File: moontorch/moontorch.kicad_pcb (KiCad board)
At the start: 2 copper layers, 24.5 x 101 mm, 27 parts, among them J1 Conn_Coaxial, J2 Pogo_VLED_1, J3 Pogo_VLED_2, J4 BAT, J5 Torchbutton, J6 UART, J7 USB, J8 Pogo_GND, Q1 AP2317SD, SW3 RESET, SW4 BOOT, U1 HT-CT62, U2 L80-R, U3 XTX XTP2038-330AS2CT

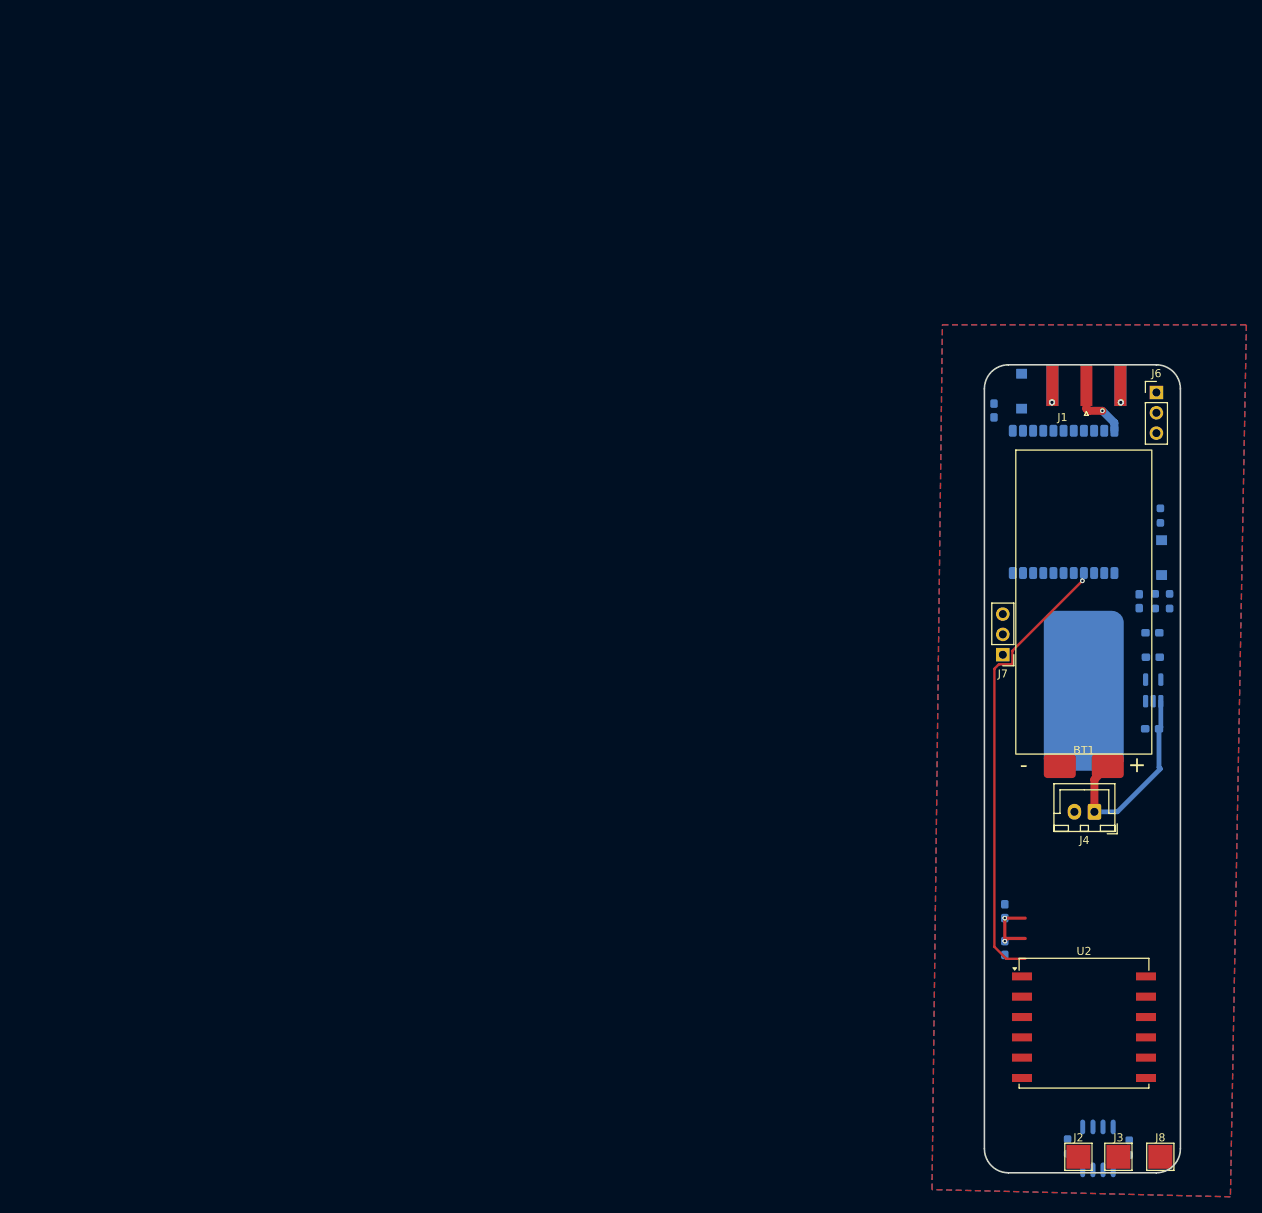
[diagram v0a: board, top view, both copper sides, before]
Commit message: weiter moontorch
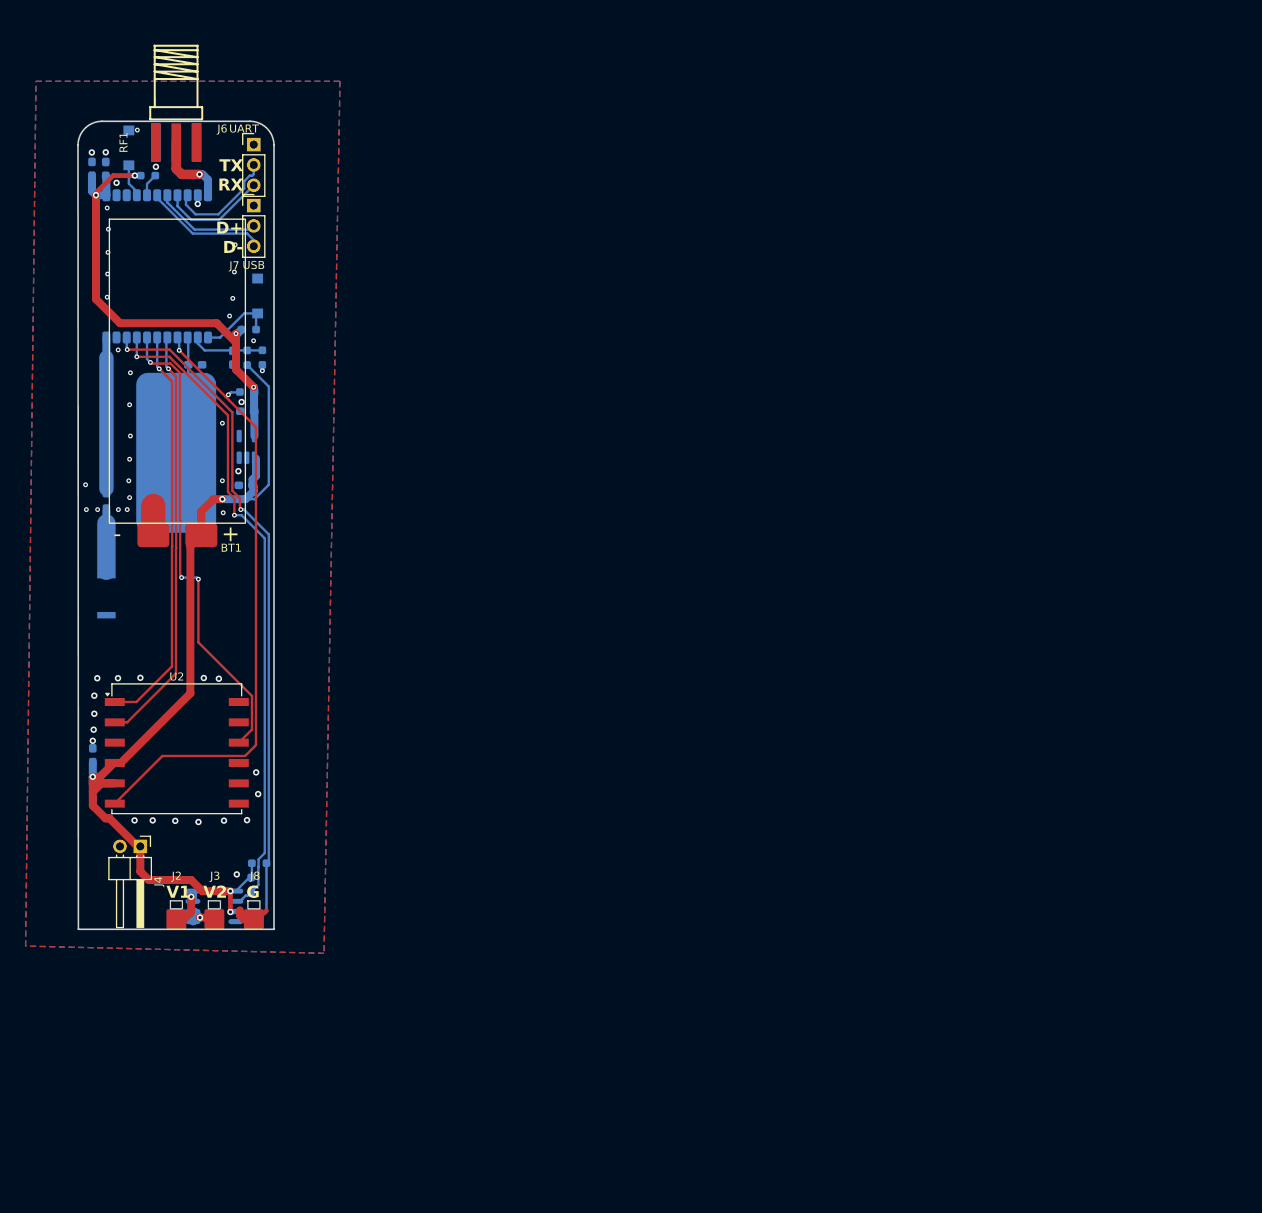
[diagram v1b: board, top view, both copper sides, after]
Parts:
- removed J1: Conn_Coaxial, Connector_Coaxial:SMA_Amphenol_132289_EdgeMount
- added C8: 1u, Capacitor_SMD:C_0603_1608Metric_Pad1.08x0.95mm_HandSolder, B.Cu at (103.4, 33.5)
- added R6: 0R, Resistor_SMD:R_0603_1608Metric_Pad0.98x0.95mm_HandSolder, B.Cu at (103.5, 75.0)
- added R8: 10K, Resistor_SMD:R_0603_1608Metric_Pad0.98x0.95mm_HandSolder, B.Cu at (108.7, 34.4)
- added R9: 10K, Resistor_SMD:R_0603_1608Metric_Pad0.98x0.95mm_HandSolder, B.Cu at (121.1, 61.4)
- added RF1: 443MHz, EasyEDA:SMA-SMD_BWSMA-KE-P001, F.Cu at (112.2, 30.2)
- added U4: 2.4GHz, EasyEDA:ANT-SMD_L5.0-W2.0, B.Cu at (103.5, 86.8)
- J2, J3, J8: footprint TestPoint:TestPoint_Pad_3.0x3.0mm -> hacrafu:Pogo Pin 3015
- J4: footprint Connector_JST:JST_XH_B2B-XH-A_1x02_P2.50mm_Vertical -> Connector_PinHeader_2.54mm:PinHeader_1x02_P2.54mm_Horizontal
- moved C7 124.3 mm to (114.6, 58.0), turned to 0 degrees
- moved R3 120.0 mm to (121.3, 53.6), turned to 180 degrees
- moved J4 119.3 mm to (107.7, 118.2), turned to -90 degrees
- moved U2 118.5 mm to (112.3, 106.0)
- moved SW3 117.6 mm to (122.4, 49.4)
- moved R4 117.5 mm to (121.1, 57.1)
- moved J8 117.5 mm to (121.9, 126.0)
- moved C1 117.3 mm to (120.9, 73.1)
- moved C3 117.3 mm to (119.3, 57.1)
- moved U3 117.3 mm to (121.0, 68.3)
- moved C2 117.3 mm to (121.1, 63.8)
- moved J5 117.3 mm to (112.2, 69.0)
- moved J3 117.2 mm to (117.0, 126.0)
- moved U1 117.1 mm to (109.8, 45.7)
- moved J6 117.0 mm to (121.9, 30.5)
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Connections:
- net Net-(J6-Pin_2) renamed /UART_TX
- net Net-(J6-Pin_3) renamed /UART_RX
- J7 pad 2: Net-(J7-Pin_2) -> /USB_DP
- J7 pad 3: Net-(J7-Pin_3) -> /USB_DN
- U1 pad 1: unconnected-(U1-2.4G_Ant-Pad1) -> Net-(U1-2.4G_Ant)
- U1 pad 16: unconnected-(U1-GPIO8-Pad16) -> Net-(U1-GPIO8)
- U1 pad 17: Net-(J7-Pin_2) -> /USB_DN
- U1 pad 18: Net-(J7-Pin_3) -> /USB_DP
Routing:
- net /LED2: track 0.00 -> 86.8 mm, vias 0 -> 2
- net /VBAT: track 33.6 -> 118.3 mm, vias 2 -> 4
- net /LED1: track 0.00 -> 82.0 mm, vias 0 -> 2
- net +3V3: track 0.00 -> 60.7 mm, vias 0 -> 4
- net /GPS_RESET: track 0.00 -> 59.4 mm, vias 0 -> 3
- net /GPS_TX: track 0.00 -> 52.7 mm, vias 0 -> 1
- net /GPS_RX: track 0.00 -> 50.9 mm, vias 0 -> 1
- net /GPS_PPS: track 56.6 -> 77.7 mm, vias 1 -> 2
- net Net-(U1-2.4G_Ant): track 0.00 -> 18.9 mm
- net /USB_DN: track 0.00 -> 15.4 mm
- net Net-(J5-Pin_1): track 0.00 -> 15.1 mm
- net /UART_TX: track 0.00 -> 14.0 mm
- net /UART_RX: track 0.00 -> 13.4 mm
- net /USB_DP: track 0.00 -> 13.3 mm
- net /RESET: track 0.00 -> 9.54 mm
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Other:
- outline, holes or cut-outs redrawn
- board text added: "D+ D-"
- board text added: "G"
- board text added: "TX RX"
- board text added: "V1"
- board text added: "V2"

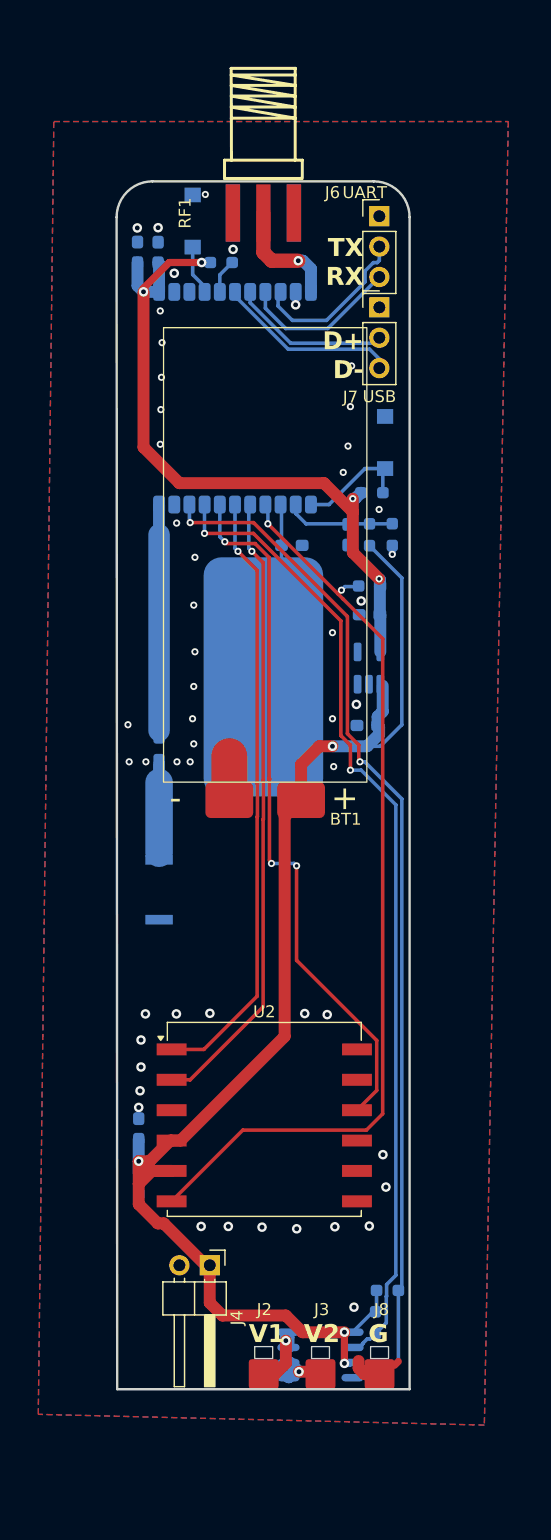
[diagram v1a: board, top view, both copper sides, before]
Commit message: zwischenstand bestellfähig 1
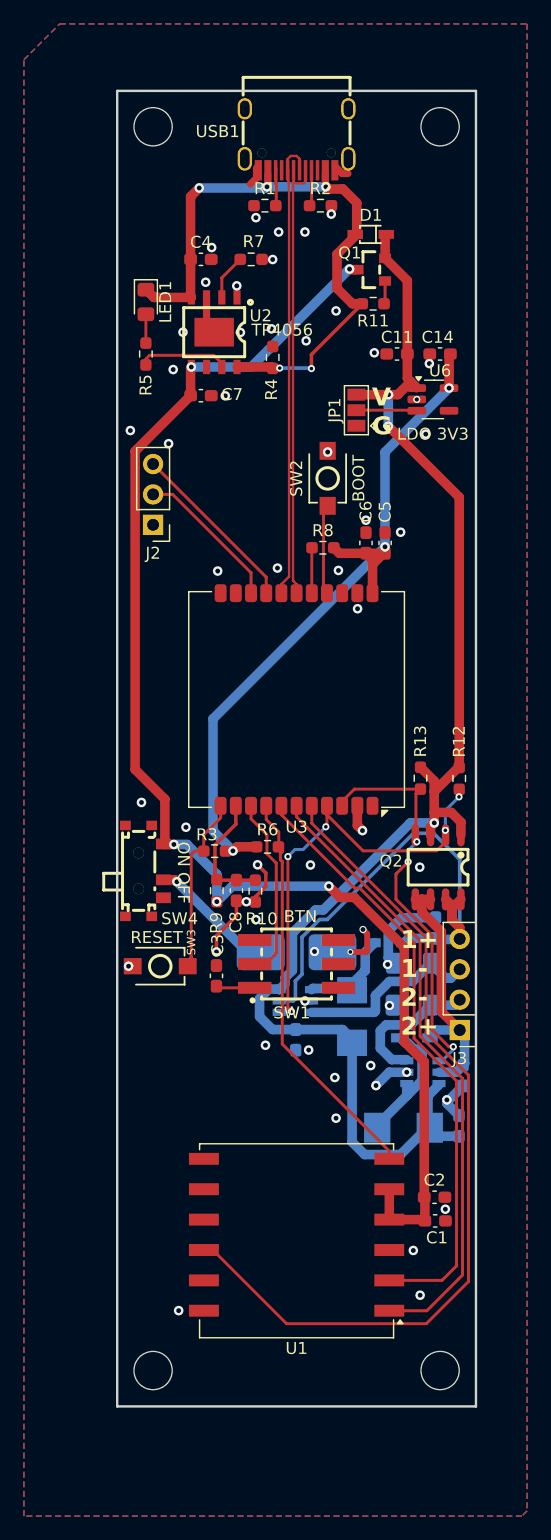
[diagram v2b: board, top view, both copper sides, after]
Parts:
- removed BT1: Battery, hacrafu:Battery 230525
- removed J4: BAT, Connector_PinHeader_2.54mm:PinHeader_1x02_P2.54mm_Horizontal
- removed J5: Torchbutton, hacrafu:Tochbutton GND
- removed J6: UART, Connector_PinHeader_2.54mm:PinHeader_1x03_P2.54mm_Vertical
- removed J7: USB, Connector_PinHeader_2.54mm:PinHeader_1x03_P2.54mm_Vertical
- removed J8: Pogo_GND, hacrafu:Pogo Pin 3015
- removed RF1: 443MHz, EasyEDA:SMA-SMD_BWSMA-KE-P001
- added C10: 1u, Capacitor_SMD:C_0603_1608Metric_Pad1.08x0.95mm_HandSolder, B.Cu at (128.6, 106.5)
- added C11: 1u, Capacitor_SMD:C_0603_1608Metric_Pad1.08x0.95mm_HandSolder, F.Cu at (123.4, 42.0)
- added C12: 1u, Capacitor_SMD:C_0603_1608Metric_Pad1.08x0.95mm_HandSolder, B.Cu at (126.6, 90.0)
- added C13: 1u, Capacitor_SMD:C_0603_1608Metric_Pad1.08x0.95mm_HandSolder, B.Cu at (128.9, 102.3)
- added C14: 1u, Capacitor_SMD:C_0603_1608Metric_Pad1.08x0.95mm_HandSolder, F.Cu at (127.0, 42.0)
- added C9: 1u, Capacitor_SMD:C_0603_1608Metric_Pad1.08x0.95mm_HandSolder, B.Cu at (114.9, 99.3)
- added D1: Schtky, EasyEDA:SOD-323_L1.8-W1.3-LS2.5-RD, F.Cu at (121.2, 32.0)
- added D2: Schtky, EasyEDA:SOD-323_L1.8-W1.3-LS2.5-RD, B.Cu at (122.7, 91.2)
- added D3: Schtky, EasyEDA:SOD-323_L1.8-W1.3-LS2.5-RD, B.Cu at (124.8, 99.2)
- added J1: BAT, hacrafu:Battery 230525, B.Cu at (115.0, 90.5)
- added JP1: SolderJumper_3_Open, Jumper:SolderJumper-3_P1.3mm_Open_Pad1.0x1.5mm, F.Cu at (120.0, 46.7)
- added L1: 10u, EasyEDA:IND-SMD_L5.4-W5.2_FXL0530, B.Cu at (119.6, 97.4)
- added L2: 10u, EasyEDA:IND-SMD_L5.4-W5.2_FXL0530, B.Cu at (123.9, 106.7)
- added LED1: CHRG, LED_SMD:LED_0805_2012Metric_Pad1.15x1.40mm_HandSolder, F.Cu at (102.4, 37.6)
- added Q2: AP2317SD, EasyEDA:SOP-8_L4.9-W3.9-P1.27-LS6.0-BL, F.Cu at (126.8, 84.9)
- added R10: 100K, Resistor_SMD:R_0603_1608Metric_Pad0.98x0.95mm_HandSolder, F.Cu at (111.5, 86.9)
- added R11: 1k, Resistor_SMD:R_0603_1608Metric_Pad0.98x0.95mm_HandSolder, F.Cu at (121.4, 37.8)
- added R12: 10K, Resistor_SMD:R_0603_1608Metric_Pad0.98x0.95mm_HandSolder, F.Cu at (128.6, 77.5)
- added R13: 10K, Resistor_SMD:R_0603_1608Metric_Pad0.98x0.95mm_HandSolder, F.Cu at (125.4, 77.5)
- added R14: 0R5, Resistor_SMD:R_1206_3216Metric_Pad1.30x1.75mm_HandSolder, B.Cu at (124.7, 92.9)
- added R15: 0R5, Resistor_SMD:R_1206_3216Metric_Pad1.30x1.75mm_HandSolder, B.Cu at (124.7, 96.5)
- added R7: 1k5, Resistor_SMD:R_0603_1608Metric_Pad0.98x0.95mm_HandSolder, F.Cu at (111.2, 34.1)
- added REF**: MountingHole_3.2mm_M3, MountingHole:MountingHole_3.2mm_M3, F.Cu at (127.0, 127.0)
- added REF**: MountingHole_3.2mm_M3, MountingHole:MountingHole_3.2mm_M3, F.Cu at (103.0, 23.0)
- added REF**: MountingHole_3.2mm_M3, MountingHole:MountingHole_3.2mm_M3, F.Cu at (127.0, 23.0)
- added REF**: MountingHole_3.2mm_M3, MountingHole:MountingHole_3.2mm_M3, F.Cu at (103.0, 127.0)
- added SW1: BTN, EasyEDA:SW-SMD_6P-L5.8-W5.8-P2.00-LS8.5-TR, F.Cu at (115.0, 93.0)
- added SW2: BOOT, EasyEDA:SW-SMD_L3.9-W3.0-P4.45, F.Cu at (117.6, 52.4)
- added U5: MT9201, EasyEDA:SOT-23-6_L2.9-W1.6-P0.95-LS2.8-BR, B.Cu at (125.6, 102.1)
- added U6: LDO 3V3, Package_TO_SOT_SMD:SOT-23-5_HandSoldering, F.Cu at (126.4, 45.8)
- added USB1: USB-TYPE-C-018, EasyEDA:USB-C_SMD-TYPE-C-31-M-12, F.Cu at (115.0, 24.0)
- C1, C7: value 1u -> 10u; moved to F.Cu
- C2, C8: value 1u -> 100n; moved to F.Cu
- C3: value 100n -> 1u; moved to F.Cu
- C4: value 100n -> 10u; moved to F.Cu
- C5: value 10u -> 1u; moved to F.Cu
- C6, R3, R8, SW3: moved to F.Cu
- J2: value Pogo_VLED_1 -> UART; footprint hacrafu:Pogo Pin 3015 -> Connector_PinHeader_2.54mm:PinHeader_1x03_P2.54mm_Vertical
- J3: value Pogo_VLED_2 -> LED; footprint hacrafu:Pogo Pin 3015 -> Connector_PinHeader_2.54mm:PinHeader_1x04_P2.54mm_Vertical
- Q1: value AP2317SD -> AO3401A; footprint EasyEDA:SOP-8_L4.9-W3.9-P1.27-LS6.0-BL -> EasyEDA:SOT-23_L2.9-W1.3-P1.90-LS2.4-BR; moved to F.Cu
- R1, R2: value 10K -> 5k1; moved to F.Cu
- R4: value 100K -> 10K; moved to F.Cu
- R5: value 100K -> 330; moved to F.Cu
- R6: value 0R -> 10K; moved to F.Cu
- R9: value 10K -> 100K; moved to F.Cu
- SW4: value BOOT -> ON OFF; footprint EasyEDA:SW-SMD_L3.9-W3.0-P4.45 -> EasyEDA:SW-TH_K3-1296S-E1; moved to F.Cu
- U1: value HT-CT62 -> L80-R; footprint RF_Module:Heltec_HT-CT62 -> RF_GPS:Quectel_L80-R; moved to F.Cu
- U2: value L80-R -> TP4056; footprint RF_GPS:Quectel_L80-R -> EasyEDA:ESOP-8_L4.9-W3.9-P1.27-LS6.0-BL-EP
- U3: value XTX XTP2038-330AS2CT -> HT-CT62; footprint Package_TO_SOT_SMD:SOT-23-5_HandSoldering -> RF_Module:Heltec_HT-CT62; moved to F.Cu
- U4: value 2.4GHz -> MT9201; footprint EasyEDA:ANT-SMD_L5.0-W2.0 -> EasyEDA:SOT-23-6_L2.9-W1.6-P0.95-LS2.8-BR
- moved R1 93.9 mm to (112.3, 29.6), turned to 0 degrees
- moved R2 90.9 mm to (117.0, 29.6)
- moved Q1 90.8 mm to (121.2, 35.0), turned to 0 degrees
- moved C4 72.9 mm to (107.0, 34.1), turned to 0 degrees
- moved U1 70.6 mm to (115.0, 116.2), turned to 180 degrees
- moved J2 70.3 mm to (103.0, 56.3), turned to 180 degrees
- moved U2 66.0 mm to (108.1, 40.2), turned to 180 degrees
- moved C5 57.4 mm to (122.4, 57.8), turned to 90 degrees
- moved SW4 54.5 mm to (102.3, 85.2), turned to 0 degrees
- moved C8 53.7 mm to (110.0, 86.9), turned to -90 degrees
- moved C2 49.0 mm to (126.5, 112.5), turned to 0 degrees
- moved SW3 47.7 mm to (103.6, 93.2), turned to 180 degrees
- moved C1 41.8 mm to (126.6, 114.5), turned to 0 degrees
- moved C3 38.5 mm to (108.3, 94.0), turned to 90 degrees
- moved R3 32.7 mm to (108.2, 83.6), turned to 0 degrees
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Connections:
- C2 pad 1: +3V3 -> /VBAT
- C3 pad 1: /BAT_SENS -> Net-(C3-Pad1)
- C4 pad 1: /VBAT -> /5V
- C5 pad 1: /VBAT -> +3V3
- C7 pad 1: Net-(J5-Pin_1) -> /VBAT
- C8 pad 1: +3V3 -> /BAT_SENS
- J2 pad 1: /VLED1 -> GND
- J3 pad 1: /VLED2 -> /LED2_A
- Q1 pad 1: /VBAT -> Net-(Q1-G)
- Q1 pad 2: /LED1 -> /VBUS
- R1 pad 1: /VBAT -> GND
- R1 pad 2: /LED1 -> Net-(USB1-CC2)
- R2 pad 1: /VBAT -> Net-(USB1-CC1)
- R2 pad 2: /LED2 -> GND
- R4 pad 1: /VBAT -> /5V
- R4 pad 2: /BAT_SENS -> GND
- R5 pad 1: /BAT_SENS -> Net-(LED1--)
- R5 pad 2: GND -> Net-(U2-~{CHRG})
- R6 pad 1: Net-(U4-ANT) -> +3V3
- R6 pad 2: Net-(U1-2.4G_Ant) -> /GPS_PPS
- R8 pad 1: Net-(U1-GPIO8) -> Net-(U3-GPIO8)
- R9 pad 1: +3V3 -> /VBAT
- R9 pad 2: /GPS_PPS -> /BAT_SENS
- SW4 pad 1: /BOOT -> unconnected-(SW4-Pad1)
- SW4 pad 2: GND -> /VBAT_PRE
- U1 pad 1: Net-(U1-2.4G_Ant) -> /GPS_RX
- U1 pad 10: /BAT_SENS -> /GPS_RESET
- U1 pad 11: /RESET -> unconnected-(U1-RESERVED-Pad11)
- U1 pad 12: +3V3 -> GND
- U1 pad 2: GND -> /GPS_TX
- U1 pad 3: /LED2 -> GND
- U1 pad 4: /LED1 -> /VBAT
- U1 pad 5: /GPS_RESET -> /VBAT
- U1 pad 6: /GPS_RX -> /GPS_PPS
- U1 pad 7: /GPS_TX -> unconnected-(U1-RESERVED-Pad7)
- U1 pad 8: /GPS_PPS -> unconnected-(U1-RESERVED-Pad8)
- U1 pad 9: Net-(J5-Pin_1) -> unconnected-(U1-NC-Pad9)
- U2 pad 1: /GPS_RX -> GND
- U2 pad 2: /GPS_TX -> Net-(U2-PROG)
- U2 pad 4: /VBAT -> /5V
- U2 pad 6: /GPS_PPS -> unconnected-(U2-~{STDBY}-Pad6)
- U2 pad 7: unconnected-(U2-RESERVED-Pad7) -> Net-(U2-~{CHRG})
- U2 pad 8: unconnected-(U2-RESERVED-Pad8) -> /5V
- U2 pad 9: unconnected-(U2-NC-Pad9) -> GND
- U3 pad 1: /VBAT -> unconnected-(U3-2.4G_Ant-Pad1)
- U3 pad 3: GND -> /LED2
- U3 pad 4: unconnected-(U3-BP-Pad4) -> /LED1
- U3 pad 5: +3V3 -> /GPS_RESET
- U4 pad 1: Net-(U4-ANT) -> Net-(D2-A)
- U4 pad 2: unconnected-(U4-Pad2) -> GND
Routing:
- net /VBUS: track 0.00 -> 121.5 mm, vias 0 -> 3
- net /LED2: track 86.8 -> 33.3 mm, vias 2 -> 3
- net /5V: track 0.00 -> 53.3 mm, vias 0 -> 5
- net /LED1: track 82.0 -> 37.2 mm, vias 2 -> 5
- net /GPS_PPS: track 77.7 -> 33.9 mm, vias 2 -> 0
- net /LED1_A: track 0.00 -> 42.2 mm
- net GND: track 9.29 -> 36.5 mm, vias 52 -> 56
- net /USB_DP: track 13.3 -> 38.6 mm
- net /USB_DN: track 15.4 -> 38.4 mm
- net /LED2_A: track 0.00 -> 21.8 mm
- net Net-(U1-2.4G_Ant): track 18.9 -> 0.00 mm
- net /LED1_C: track 0.00 -> 15.7 mm
- net /BTN: track 0.00 -> 15.4 mm
- net Net-(J5-Pin_1): track 15.1 -> 0.00 mm
- net /GPS_RESET: track 59.4 -> 71.3 mm, vias 3 -> 0
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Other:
- board size 24.5 x 101 mm -> 30 x 110 mm
- board text added: "1+ 1- 2- 2+"
- board text added: "V G"
- board text removed: "D+ D-"
- board text removed: "G"
- board text removed: "TX RX"
- board text removed: "V1"
- board text removed: "V2"
